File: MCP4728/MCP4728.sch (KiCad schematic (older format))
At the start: 17 parts, among them J1 Conn_01x06, J2 Conn_01x04, J3 Conn_01x06, J4 Conn_01x04, U1 MCP4728

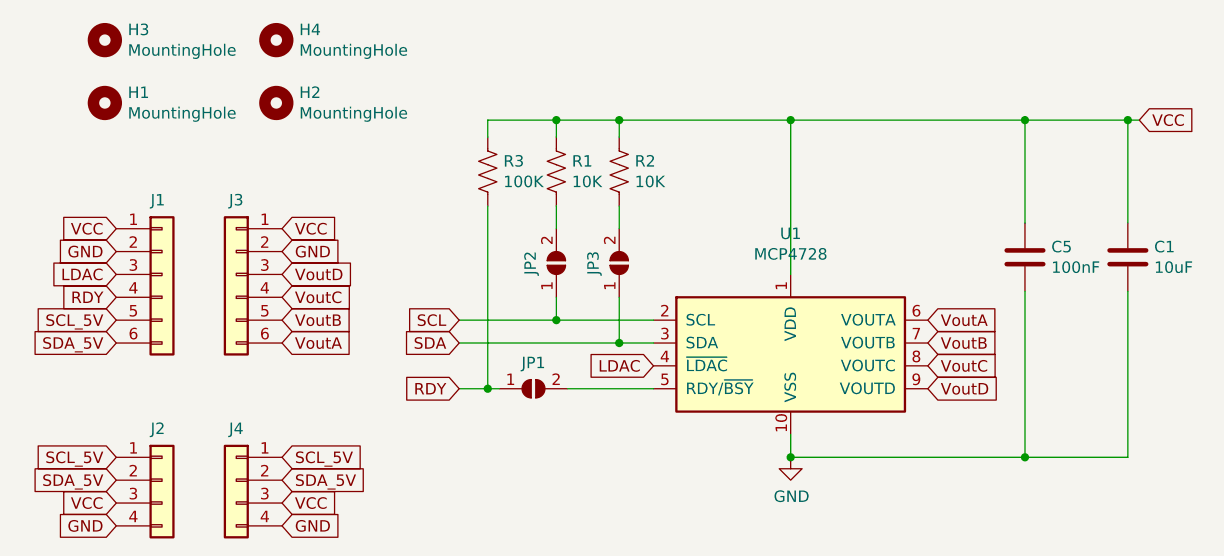
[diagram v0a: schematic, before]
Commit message: Phew...
almost a screw up
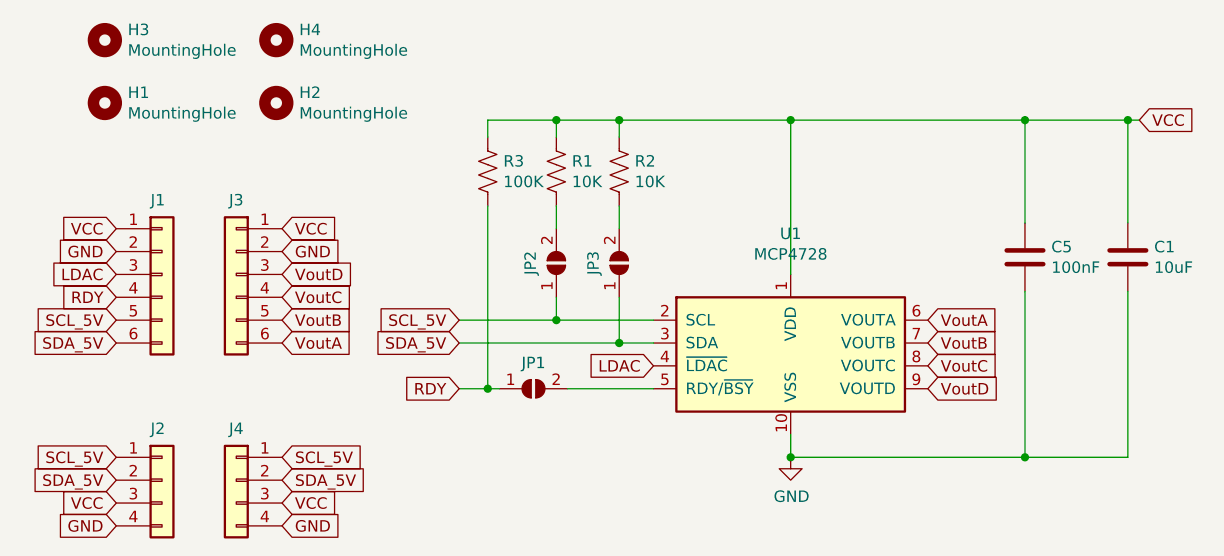
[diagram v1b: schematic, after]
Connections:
- net SCL is gone; now on net SCL_5V: JP2.1 (A), U1.2 (SCL)
- net SDA is gone; now on net SDA_5V: JP3.1 (A), U1.3 (SDA)
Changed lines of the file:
@@
 Sheet 1 1
 Title "MCP4728 Breakout "
-Date "2020-01-23"
-Rev "2"
+Date "2020-03-10"
+Rev "3"
 Comp "SirBoard"
 Comment1 "4 Channel I2C DAC with 12 Bit Resolution"
@@
 	1    0    0    -1
 $EndComp
-Text GLabel 2500 2300 0    50   Input ~ 0
-SDA
-Text GLabel 2500 2200 0    50   Input ~ 0
-SCL
 $Comp
 L Device:R_US R2
@@
 Wire Wire Line
 	3950 1325 4975 1325
+Text GLabel 2500 2300 0    50   Input ~ 0
+SDA_5V
+Text GLabel 2500 2200 0    50   Input ~ 0
+SCL_5V
 $EndSCHEMATC

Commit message: Auto stash before revert of "Board Revision"
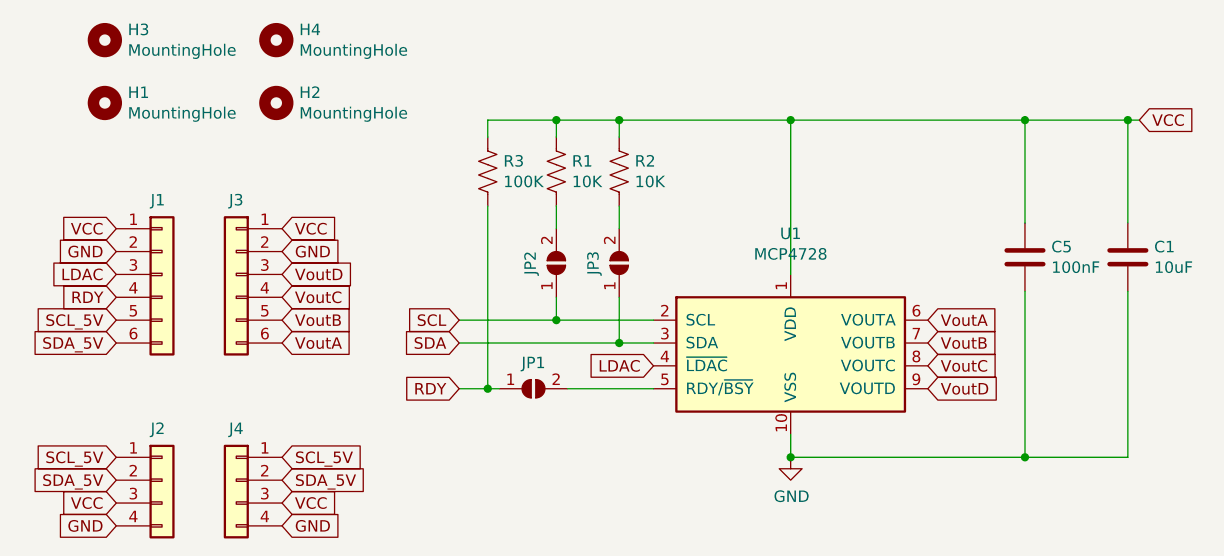
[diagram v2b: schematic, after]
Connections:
- net SCL_5V: no longer JP2.1 (A), U1.2 (SCL)
- net SDA_5V: no longer JP3.1 (A), U1.3 (SDA)
- new net SCL: JP2.1 (A), U1.2 (SCL)
- new net SDA: JP3.1 (A), U1.3 (SDA)
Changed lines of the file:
@@
 Sheet 1 1
 Title "MCP4728 Breakout "
-Date "2020-03-10"
-Rev "3"
+Date "2020-01-23"
+Rev "2"
 Comp "SirBoard"
 Comment1 "4 Channel I2C DAC with 12 Bit Resolution"
@@
 	1    0    0    -1
 $EndComp
+Text GLabel 2500 2300 0    50   Input ~ 0
+SDA
+Text GLabel 2500 2200 0    50   Input ~ 0
+SCL
 $Comp
 L Device:R_US R2
@@
 Wire Wire Line
 	3950 1325 4975 1325
-Text GLabel 2500 2300 0    50   Input ~ 0
-SDA_5V
-Text GLabel 2500 2200 0    50   Input ~ 0
-SCL_5V
 $EndSCHEMATC
